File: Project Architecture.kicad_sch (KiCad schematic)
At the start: 0 parts

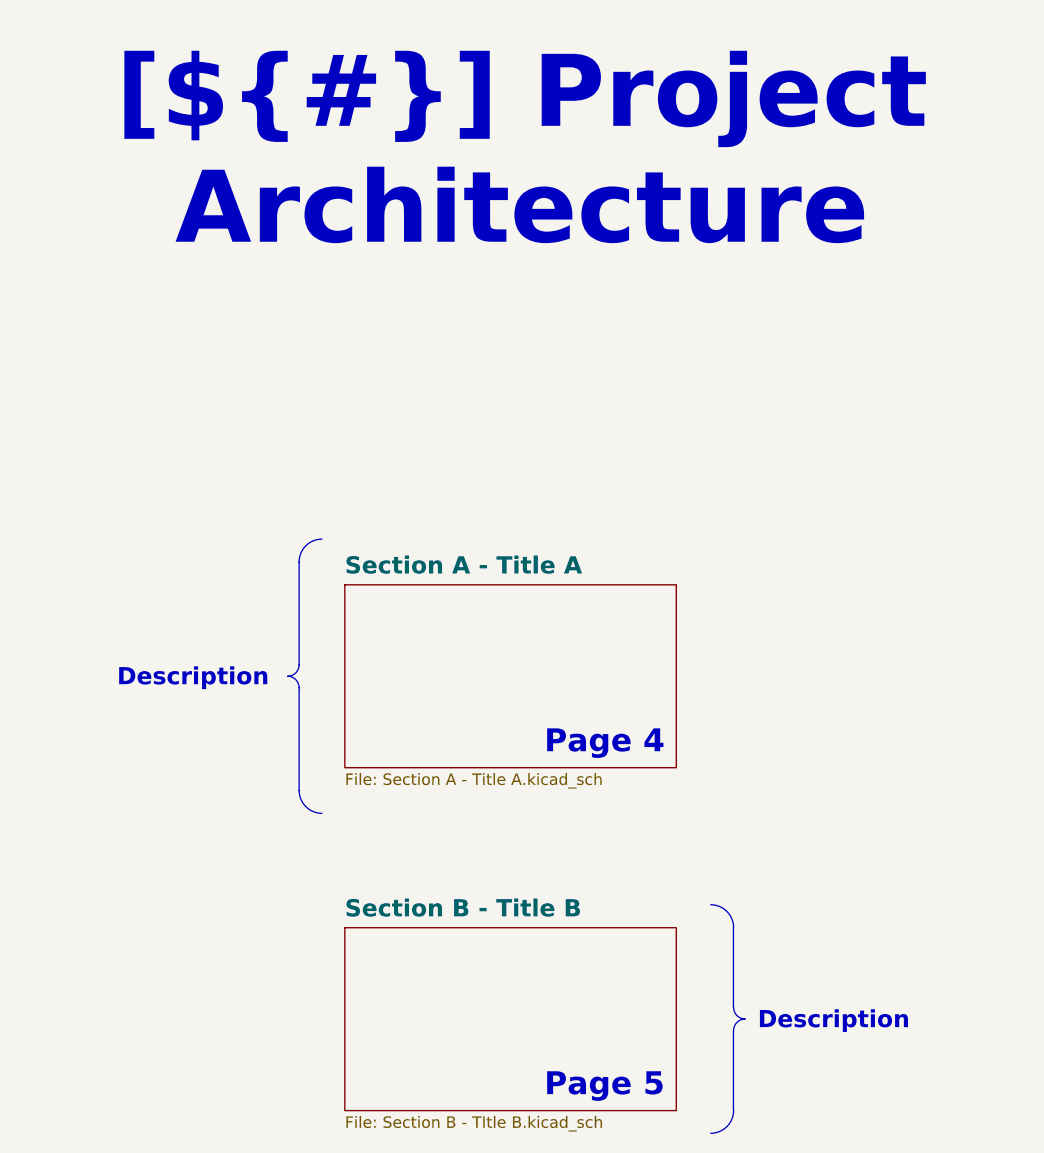
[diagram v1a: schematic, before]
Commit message: test ;
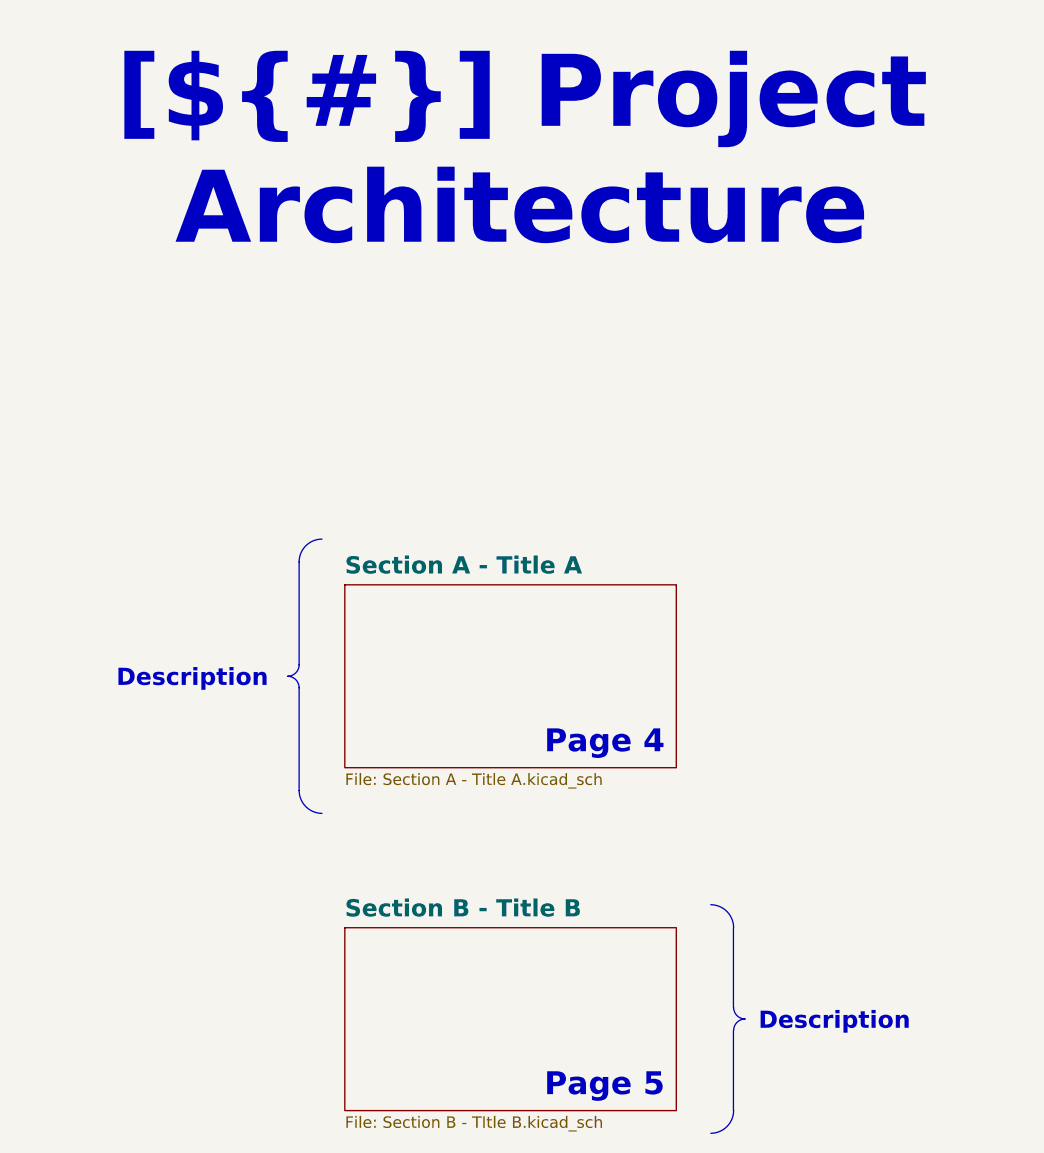
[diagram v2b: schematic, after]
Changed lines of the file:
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@@
 (kicad_sch
-	(version 20260306)
+	(version 20231120)
 	(generator "eeschema")
-	(generator_version "10.0")
+	(generator_version "8.0")
 	(paper "A3")
 	(title_block
@@
 		(company "${COMPANY}")
 	)
+	(polyline
+		(pts
+			(xy 185.42 87.63) (xy 185.42 99.06)
+		)
+		(stroke
+			(width 0)
+			(type default)
+		)
+	)
+	(polyline
+		(pts
+			(xy 233.68 125.73) (xy 233.68 134.62)
+		)
+		(stroke
+			(width 0)
+			(type default)
+		)
+	)
+	(polyline
+		(pts
+			(xy 185.42 85.09) (xy 185.42 73.66)
+		)
+		(stroke
+			(width 0)
+			(type default)
+		)
+	)
+	(polyline
+		(pts
+			(xy 233.68 114.3) (xy 233.68 123.19)
+		)
+		(stroke
+			(width 0)
+			(type default)
+		)
+	)
 	(arc
 		(start 185.42 85.09)
@@
 		)
 	)
-	(text "Page 5"
-		(exclude_from_sim no)
-		(at 226.06 133.35 0)
-		(effects
-			(font
-				(size 2.54 2.54)
-				(bold yes)
-				(color 100 70 50 1)
-			)
-			(justify right bottom)
-			(href "#5")
-		)
-	)
-	(text "Page 4"
-		(exclude_from_sim no)
-		(at 226.06 95.25 0)
-		(effects
-			(font
-				(size 2.54 2.54)
-				(bold yes)
-				(color 20 60 40 1)
-			)
-			(justify right bottom)
-			(href "#4")
-		)
-	)
 	(text_box "Description"
 		(exclude_from_sim no)
 		(at 166.37 83.82 0)
 		(size 17.145 5.08)
-		(margins 1.4287 1.4287 1.4287 1.4287)
 		(stroke
 			(width -0.0001)
@@
 		(at 234.95 121.92 0)
 		(size 26.015 5.1)
-		(margins 1.4287 1.4287 1.4287 1.4287)
 		(stroke
 			(width -0.0001)
@@
 		(at 144.78 21.59 0)
 		(size 130.81 12.7)
-		(margins 5.9999 5.9999 5.9999 5.9999)
 		(stroke
 			(width -0.0001)
@@
 		)
 	)
-	(polyline
-		(pts
-			(xy 185.42 87.63) (xy 185.42 99.06)
-		)
-		(stroke
-			(width 0)
-			(type default)
-		)
-	)
-	(polyline
-		(pts
-			(xy 233.68 125.73) (xy 233.68 134.62)
-		)
-		(stroke
-			(width 0)
-			(type default)
-		)
-	)
-	(polyline
-		(pts
-			(xy 185.42 85.09) (xy 185.42 73.66)
-		)
-		(stroke
-			(width 0)
-			(type default)
-		)
-	)
-	(polyline
-		(pts
-			(xy 233.68 114.3) (xy 233.68 123.19)
-		)
-		(stroke
-			(width 0)
-			(type default)
+	(text "Page 5"
+		(exclude_from_sim no)
+		(at 226.06 133.35 0)
+		(effects
+			(font
+				(size 2.54 2.54)
+				(bold yes)
+				(color 100 70 50 1)
+			)
+			(justify right bottom)
+			(href "#5")
+		)
+	)
+	(text "Page 4"
+		(exclude_from_sim no)
+		(at 226.06 95.25 0)
+		(effects
+			(font
+				(size 2.54 2.54)
+				(bold yes)
+				(color 20 60 40 1)
+			)
+			(justify right bottom)
+			(href "#4")
 		)
 	)
@@
 		(at 190.5 114.3)
 		(size 36.83 20.32)
-		(exclude_from_sim no)
-		(in_bom yes)
-		(on_board yes)
-		(dnp no)
 		(fields_autoplaced yes)
 		(stroke
@@
 		)
 		(fill
-			(color 255 200 0 0.502)
+			(color 255 200 0 0.5020)
 		)
 		(property "Sheetname" "Section B - Title B"
 			(at 190.5 113.2709 0)
-			(show_name no)
-			(do_not_autoplace no)
 			(effects
 				(font
@@
 		(property "Sheetfile" "Section B - TItle B.kicad_sch"
 			(at 190.5 135.2046 0)
-			(show_name no)
-			(do_not_autoplace no)
 			(effects
 				(font
@@
 		)
 		(instances
-			(project "test"
+			(project "KDT_Hierarchical_KiBot"
 				(path "/f9e05184-c88b-4a88-ae9c-ab2bdb32be7c/c5103ceb-5325-4a84-a025-9638a412984e"
 					(page "5")
@@
 		(at 190.5 76.2)
 		(size 36.83 20.32)
-		(exclude_from_sim no)
-		(in_bom yes)
-		(on_board yes)
-		(dnp no)
 		(fields_autoplaced yes)
 		(stroke
@@
 		)
 		(fill
-			(color 128 255 128 0.5)
+			(color 128 255 128 0.5000)
 		)
 		(property "Sheetname" "Section A - Title A"
 			(at 190.5 75.1709 0)
-			(show_name no)
-			(do_not_autoplace no)
 			(effects
 				(font
@@
 		(property "Sheetfile" "Section A - Title A.kicad_sch"
 			(at 190.5 97.1046 0)
-			(show_name no)
-			(do_not_autoplace no)
 			(effects
 				(font
@@
 		)
 		(instances
-			(project "test"
+			(project "KDT_Hierarchical_KiBot"
 				(path "/f9e05184-c88b-4a88-ae9c-ab2bdb32be7c/c5103ceb-5325-4a84-a025-9638a412984e"
 					(page "4")
